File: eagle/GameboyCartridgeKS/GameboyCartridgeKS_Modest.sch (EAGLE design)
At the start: 32 parts, among them IC2 MEGA64-A, Y1 16MHz max

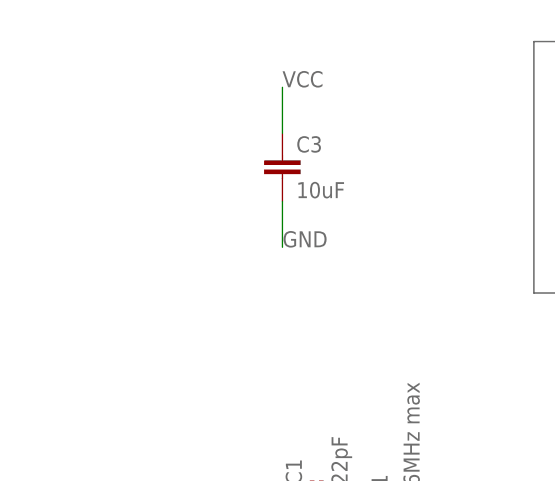
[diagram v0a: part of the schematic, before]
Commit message: Placement beta before routing
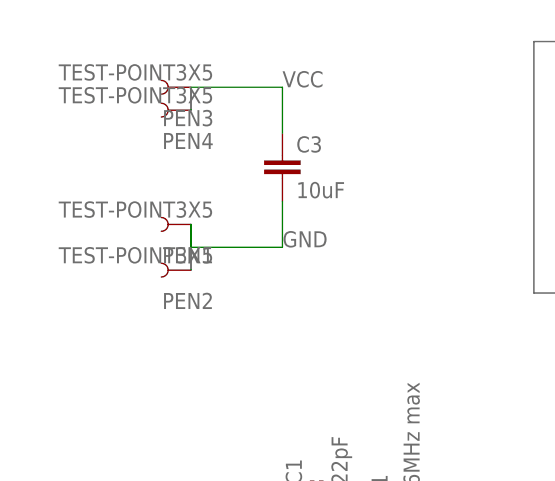
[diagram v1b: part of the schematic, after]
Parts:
- added PEN1, PEN2, PEN3, PEN4: TEST-POINT3X5, SparkFun-Passives:TEST-POINT3X5
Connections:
- net GND: now also PEN1.1, PEN2.1
- net VCC: now also PEN3.1, PEN4.1
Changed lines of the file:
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@@
 <part name="JCE_CS" library="SparkFun-Passives" deviceset="JUMPER-PAD-2-NO" device="" value=""/>
 <part name="JOE_RD" library="SparkFun-Passives" deviceset="JUMPER-PAD-2-NO" device="" value=""/>
+<part name="PEN1" library="SparkFun-Passives" deviceset="TEST-POINT" device="3X5"/>
+<part name="PEN2" library="SparkFun-Passives" deviceset="TEST-POINT" device="3X5"/>
+<part name="PEN3" library="SparkFun-Passives" deviceset="TEST-POINT" device="3X5"/>
+<part name="PEN4" library="SparkFun-Passives" deviceset="TEST-POINT" device="3X5"/>
 </parts>
 <sheets>
@@
 <instance part="JCE_CS" gate="G$1" x="185.42" y="162.56" rot="R90"/>
 <instance part="JOE_RD" gate="G$1" x="193.04" y="152.4" rot="R90"/>
+<instance part="PEN1" gate="G$1" x="-27.94" y="256.54" rot="R180"/>
+<instance part="PEN2" gate="G$1" x="-27.94" y="251.46" rot="R180"/>
+<instance part="PEN3" gate="G$1" x="-27.94" y="271.78" rot="R180"/>
+<instance part="PEN4" gate="G$1" x="-27.94" y="269.24" rot="R180"/>
 </instances>
 <busses>
@@
 <wire x1="-17.78" y1="259.08" x2="-17.78" y2="254" width="0.1524" layer="91"/>
 <label x="-17.78" y="254" size="1.778" layer="95"/>
+<pinref part="PEN1" gate="G$1" pin="1"/>
+<wire x1="-17.78" y1="254" x2="-27.94" y2="254" width="0.1524" layer="91"/>
+<wire x1="-27.94" y1="254" x2="-27.94" y2="256.54" width="0.1524" layer="91"/>
+<pinref part="PEN2" gate="G$1" pin="1"/>
+<wire x1="-27.94" y1="256.54" x2="-27.94" y2="251.46" width="0.1524" layer="91"/>
 </segment>
 <segment>
@@
 <wire x1="-17.78" y1="266.7" x2="-17.78" y2="271.78" width="0.1524" layer="91"/>
 <label x="-17.78" y="271.78" size="1.778" layer="95"/>
-</segment>
-<segment>
+<pinref part="PEN3" gate="G$1" pin="1"/>
+<wire x1="-17.78" y1="271.78" x2="-27.94" y2="271.78" width="0.1524" layer="91"/>
+<pinref part="PEN4" gate="G$1" pin="1"/>
+<wire x1="-27.94" y1="271.78" x2="-27.94" y2="269.24" width="0.1524" layer="91"/>
+</segment>
+<segment>
